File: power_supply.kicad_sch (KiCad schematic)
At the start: 31 parts

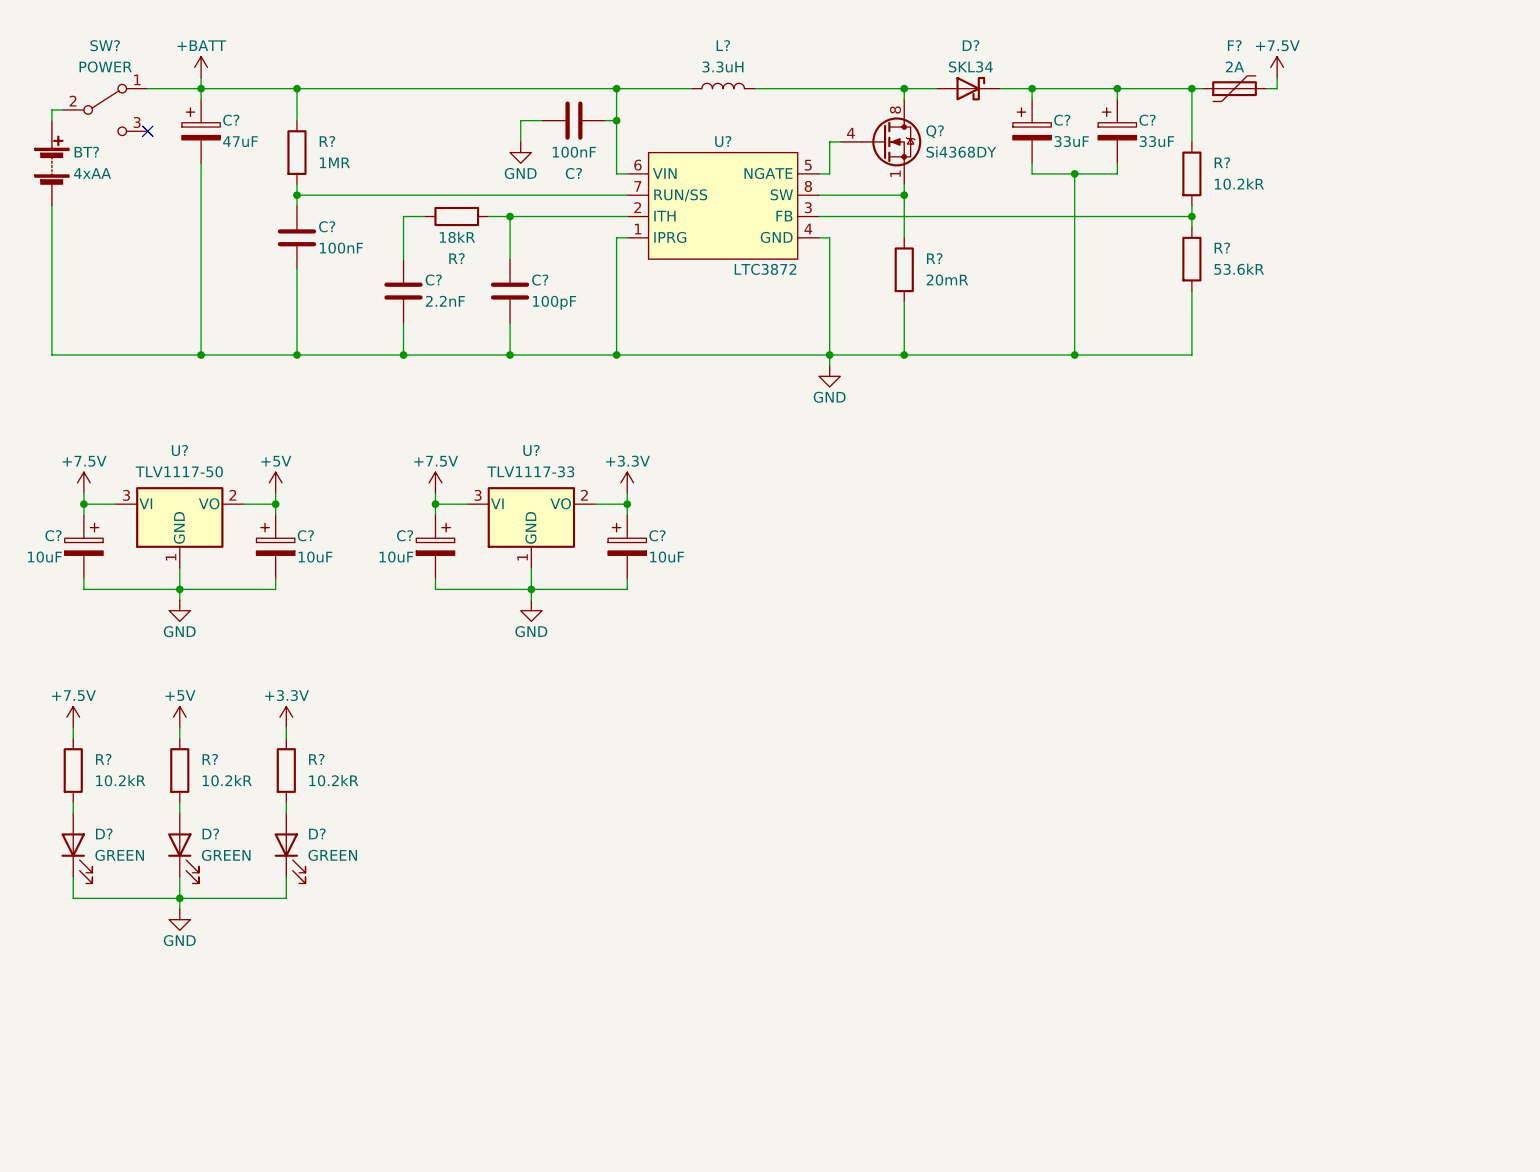
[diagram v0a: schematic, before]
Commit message: Power supply schematic beautified
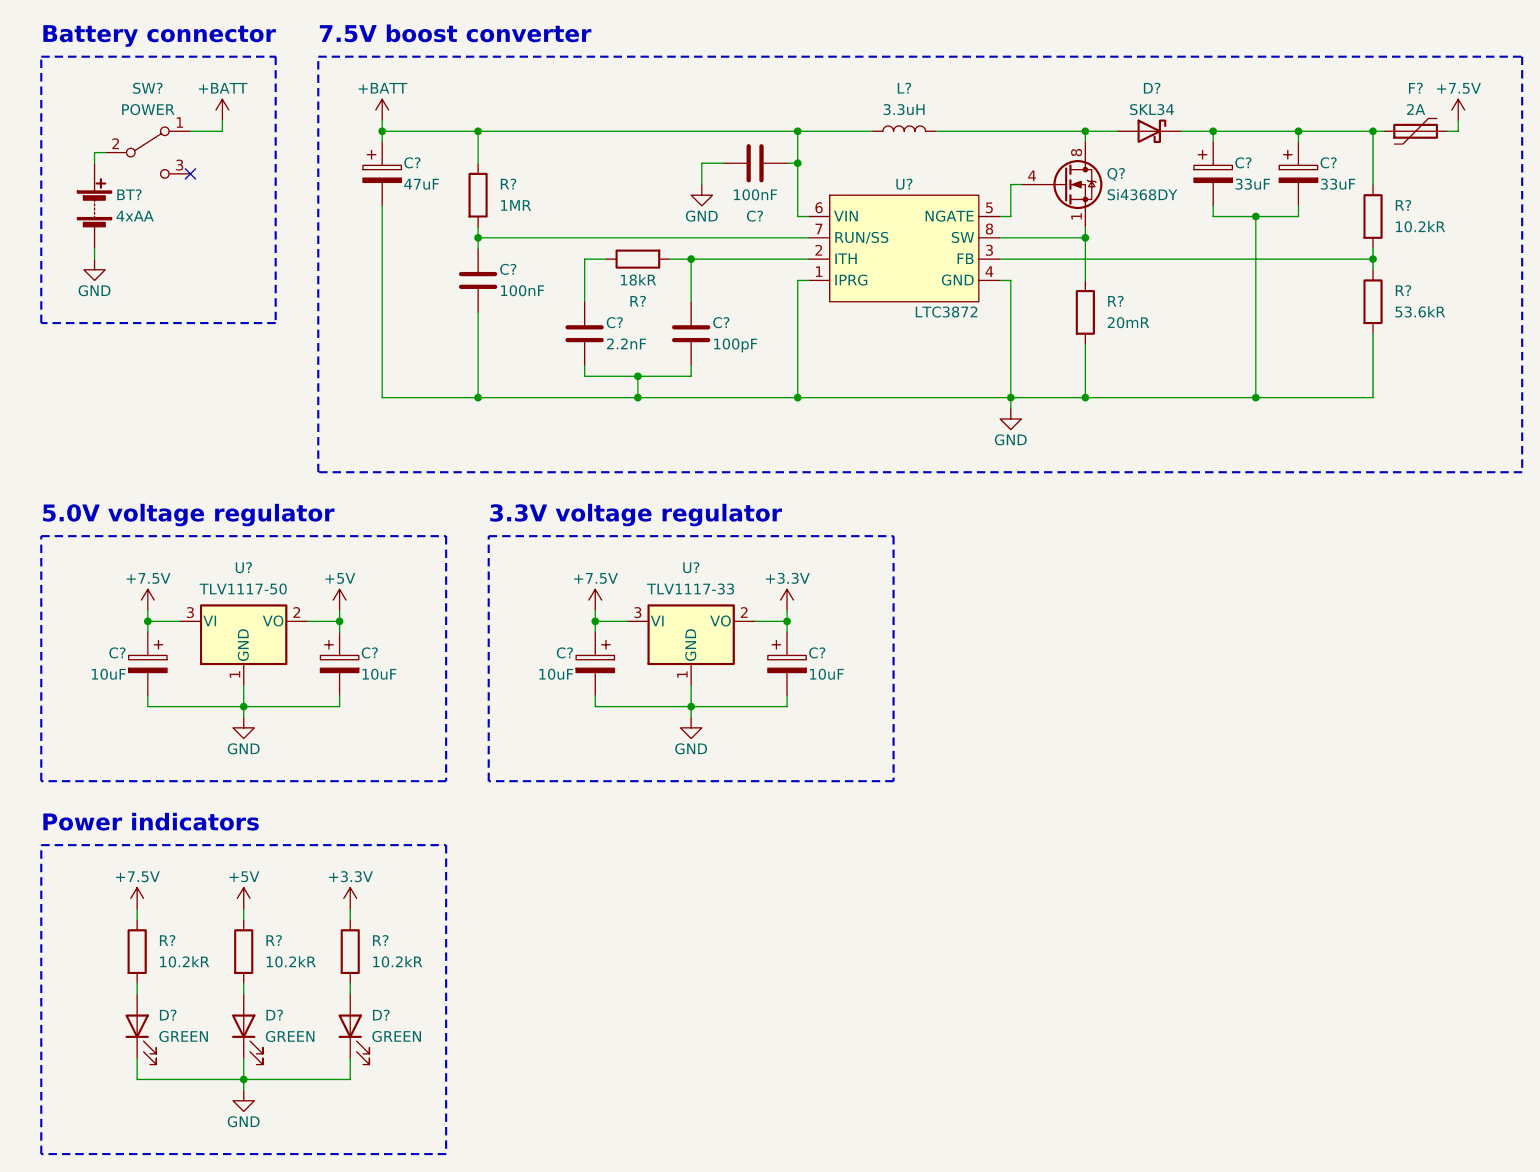
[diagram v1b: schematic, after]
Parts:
- removed BT?: 4xAA, symbol Device:Battery
- removed C? (x2): 10uF, symbol Device:C_Polarized
- removed SW?: POWER, symbol Switch:SW_SPDT
- added BT?: 4xAA, symbol Device:Battery
- added C? (x2): 10uF, symbol Device:C_Polarized
- added SW?: POWER, symbol Switch:SW_SPDT
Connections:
- net +5V: now also C?.1
- net +7.5V: now also C?.1
- net +BATT: now also SW?.1 (A)
- net GND: now also BT?.2 (-), C?.2, C?.2
- new net: BT?.1 (+), SW?.2 (B)
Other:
- note added: "3.3V voltage regulator"
- note added: "5.0V voltage regulator"
- note added: "7.5V boost converter"
- note added: "Battery connector"
- note added: "Power indicators"
- moved on the sheet: C?, D?, F?, L?, Q?, R?, U?
